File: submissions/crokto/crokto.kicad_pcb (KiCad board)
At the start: 2 copper layers, 88.9 x 50 mm, 27 parts, among them J1 USB_C_Receptacle, K1 UP, K3 LEFT, K4 RIGHT, K6 A, K7 DOWN, K8 B, SW1 SW_PUSH, SW2 SELECT, SW3 START, U1 ATmega32U2-AU, Y1 Resonator

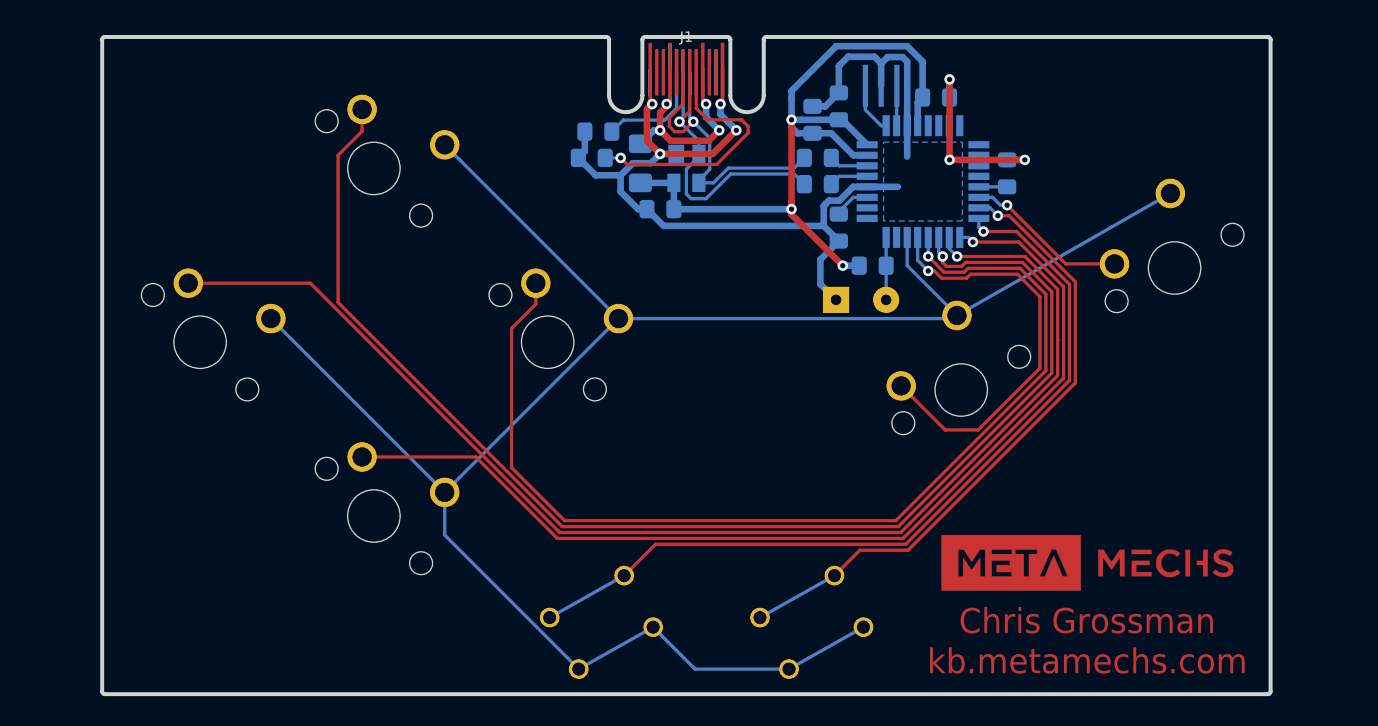
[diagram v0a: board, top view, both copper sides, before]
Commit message: switched design entirely lol
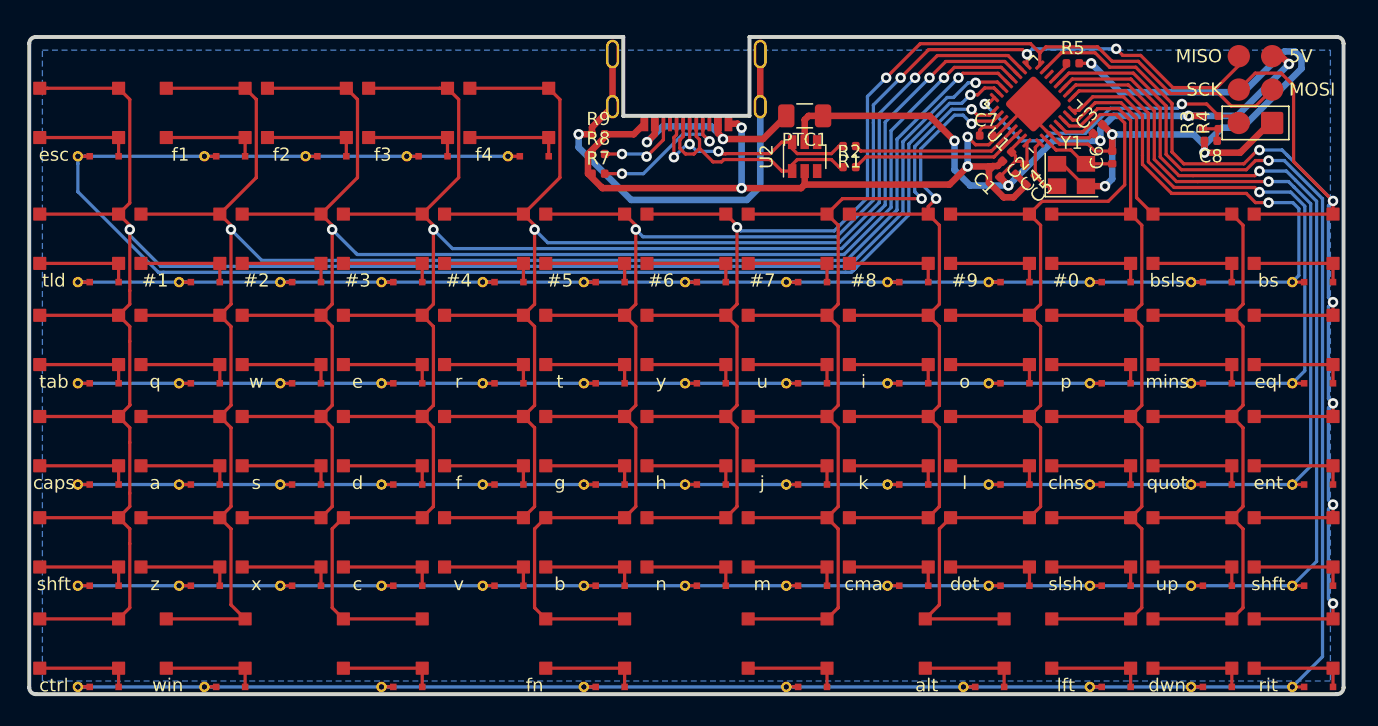
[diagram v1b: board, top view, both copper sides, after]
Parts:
- removed G***: LOGO, logo:qr
- removed L1: MountingHole, logo:new logo
- removed R6: 5.1k, Resistor_SMD:R_0805_2012Metric_Pad1.15x1.40mm_HandSolder
- removed SW1: SW_PUSH, Connector_Wire:SolderWirePad_1x02_P3.81mm_Drill0.8mm
- removed SW2: SELECT, crokto:FSMJ_2-1825910-7
- removed SW3: START, crokto:FSMJ_2-1825910-7
- added C6: 10pf, Capacitor_SMD:C_0402_1005Metric, F.Cu at (82.4, 9.16)
- added C7: 1u, Capacitor_SMD:C_0402_1005Metric, F.Cu at (72.8, 7.50)
- added C8: 100n, Capacitor_SMD:C_0402_1005Metric, F.Cu at (89.9, 7.90)
- added D10: D, crokto:D_SOD-323F-VIA, F.Cu at (36.5, 18.6)
- added D11: D, crokto:D_SOD-323F-VIA, F.Cu at (44.2, 18.6)
- added D12: D, crokto:D_SOD-323F-VIA, F.Cu at (51.9, 18.6)
- added D13: D, crokto:D_SOD-323F-VIA, F.Cu at (59.6, 18.6)
- added D14: D, crokto:D_SOD-323F-VIA, F.Cu at (67.3, 18.6)
- added D15: D, crokto:D_SOD-323F-VIA, F.Cu at (75.0, 18.6)
- added D16: D, crokto:D_SOD-323F-VIA, F.Cu at (82.7, 18.6)
- added D17: D, crokto:D_SOD-323F-VIA, F.Cu at (90.4, 18.6)
- added D18: D, crokto:D_SOD-323F-VIA, F.Cu at (98.1, 18.6)
- added D19: D, crokto:D_SOD-323F-VIA, F.Cu at (5.70, 26.4)
- added D2: D, crokto:D_SOD-323F-VIA, F.Cu at (15.3, 9.07)
- added D20: D, crokto:D_SOD-323F-VIA, F.Cu at (13.4, 26.4)
- added D21: D, crokto:D_SOD-323F-VIA, F.Cu at (21.1, 26.4)
- added D22: D, crokto:D_SOD-323F-VIA, F.Cu at (28.8, 26.4)
- added D23: D, crokto:D_SOD-323F-VIA, F.Cu at (36.5, 26.4)
- added D24: D, crokto:D_SOD-323F-VIA, F.Cu at (44.2, 26.4)
- added D25: D, crokto:D_SOD-323F-VIA, F.Cu at (51.9, 26.4)
- added D26: D, crokto:D_SOD-323F-VIA, F.Cu at (59.6, 26.4)
- added D27: D, crokto:D_SOD-323F-VIA, F.Cu at (67.3, 26.4)
- added D28: D, crokto:D_SOD-323F-VIA, F.Cu at (75.0, 26.4)
- added D29: D, crokto:D_SOD-323F-VIA, F.Cu at (82.7, 26.4)
- added D3: D, crokto:D_SOD-323F-VIA, F.Cu at (23.0, 9.07)
- added D30: D, crokto:D_SOD-323F-VIA, F.Cu at (90.4, 26.4)
- added D31: D, crokto:D_SOD-323F-VIA, F.Cu at (98.1, 26.4)
- added D32: D, crokto:D_SOD-323F-VIA, F.Cu at (5.70, 34.0)
- added D33: D, crokto:D_SOD-323F-VIA, F.Cu at (13.4, 34.0)
- added D34: D, crokto:D_SOD-323F-VIA, F.Cu at (21.1, 34.0)
- added D35: D, crokto:D_SOD-323F-VIA, F.Cu at (28.8, 34.0)
- added D36: D, crokto:D_SOD-323F-VIA, F.Cu at (36.5, 34.0)
- added D37: D, crokto:D_SOD-323F-VIA, F.Cu at (44.2, 34.0)
- added D38: D, crokto:D_SOD-323F-VIA, F.Cu at (51.9, 34.0)
- added D39: D, crokto:D_SOD-323F-VIA, F.Cu at (59.6, 34.0)
- added D4: D, crokto:D_SOD-323F-VIA, F.Cu at (30.7, 9.07)
- added D40: D, crokto:D_SOD-323F-VIA, F.Cu at (67.3, 34.0)
- added D41: D, crokto:D_SOD-323F-VIA, F.Cu at (75.0, 34.0)
- added D42: D, crokto:D_SOD-323F-VIA, F.Cu at (82.7, 34.0)
- added D43: D, crokto:D_SOD-323F-VIA, F.Cu at (90.4, 34.0)
- added D44: D, crokto:D_SOD-323F-VIA, F.Cu at (98.1, 34.0)
- added D45: D, crokto:D_SOD-323F-VIA, F.Cu at (5.70, 41.8)
- added D46: D, crokto:D_SOD-323F-VIA, F.Cu at (13.4, 41.8)
- added D47: D, crokto:D_SOD-323F-VIA, F.Cu at (21.1, 41.8)
- added D48: D, crokto:D_SOD-323F-VIA, F.Cu at (28.8, 41.8)
- added D49: D, crokto:D_SOD-323F-VIA, F.Cu at (36.5, 41.8)
- added D5: D, crokto:D_SOD-323F-VIA, F.Cu at (38.4, 9.07)
- added D50: D, crokto:D_SOD-323F-VIA, F.Cu at (44.2, 41.8)
- added D51: D, crokto:D_SOD-323F-VIA, F.Cu at (51.9, 41.8)
- added D52: D, crokto:D_SOD-323F-VIA, F.Cu at (59.6, 41.8)
- added D53: D, crokto:D_SOD-323F-VIA, F.Cu at (67.3, 41.8)
- added D54: D, crokto:D_SOD-323F-VIA, F.Cu at (75.0, 41.8)
- added D55: D, crokto:D_SOD-323F-VIA, F.Cu at (82.7, 41.8)
- added D56: D, crokto:D_SOD-323F-VIA, F.Cu at (90.4, 41.8)
- added D57: D, crokto:D_SOD-323F-VIA, F.Cu at (98.1, 41.8)
- added D58: D, crokto:D_SOD-323F-VIA, F.Cu at (5.70, 49.5)
- added D59: D, crokto:D_SOD-323F-VIA, F.Cu at (15.3, 49.5)
- added D6: D, crokto:D_SOD-323F-VIA, F.Cu at (5.70, 18.6)
- added D60: D, crokto:D_SOD-323F-VIA, F.Cu at (28.8, 49.5)
- added D61: D, crokto:D_SOD-323F-VIA, F.Cu at (44.2, 49.5)
- added D62: D, crokto:D_SOD-323F-VIA, F.Cu at (59.6, 49.5)
- added D63: D, crokto:D_SOD-323F-VIA, F.Cu at (73.1, 49.5)
- added D64: D, crokto:D_SOD-323F-VIA, F.Cu at (82.7, 49.5)
- added D65: D, crokto:D_SOD-323F-VIA, F.Cu at (90.4, 49.5)
- added D66: D, crokto:D_SOD-323F-VIA, F.Cu at (98.1, 49.5)
- added D7: D, crokto:D_SOD-323F-VIA, F.Cu at (13.4, 18.6)
- added D8: D, crokto:D_SOD-323F-VIA, F.Cu at (21.1, 18.6)
- added D9: D, crokto:D_SOD-323F-VIA, F.Cu at (28.8, 18.6)
- added H1: logo, logo:100mm wide logo, B.Cu at (51.8, 40.8)
- added H2: logo, logo:qr, B.Cu at (7.00, 7.00)
- added K10: #4, smd-keys:100, F.Cu at (34.6, 15.3)
- added K11: #5, smd-keys:100, F.Cu at (42.3, 15.3)
- added K12: #6, smd-keys:100, F.Cu at (50.0, 15.3)
- added K13: #7, smd-keys:100, F.Cu at (57.7, 15.3)
- added K14: #8, smd-keys:100, F.Cu at (65.4, 15.3)
- added K15: #9, smd-keys:100, F.Cu at (73.1, 15.3)
- added K16: #0, smd-keys:100, F.Cu at (80.8, 15.3)
- added K17: bsls, smd-keys:100, F.Cu at (88.5, 15.3)
- added K18: bs, smd-keys:100, F.Cu at (96.2, 15.3)
- added K19: tab, smd-keys:100, F.Cu at (3.80, 23.1)
- added K2: f1, smd-keys:100, F.Cu at (13.4, 5.78)
- added K20: q, smd-keys:100, F.Cu at (11.5, 23.1)
- added K21: w, smd-keys:100, F.Cu at (19.2, 23.1)
- added K22: e, smd-keys:100, F.Cu at (26.9, 23.1)
- added K23: r, smd-keys:100, F.Cu at (34.6, 23.1)
- added K24: t, smd-keys:100, F.Cu at (42.3, 23.1)
- added K25: y, smd-keys:100, F.Cu at (50.0, 23.1)
- added K26: u, smd-keys:100, F.Cu at (57.7, 23.1)
- added K27: i, smd-keys:100, F.Cu at (65.4, 23.1)
- added K28: o, smd-keys:100, F.Cu at (73.1, 23.1)
- added K29: p, smd-keys:100, F.Cu at (80.8, 23.1)
- added K30: mins, smd-keys:100, F.Cu at (88.5, 23.1)
- added K31: eql, smd-keys:100, F.Cu at (96.2, 23.1)
- added K32: caps, smd-keys:100, F.Cu at (3.80, 30.8)
- added K33: a, smd-keys:100, F.Cu at (11.5, 30.8)
- added K34: s, smd-keys:100, F.Cu at (19.2, 30.8)
- added K35: d, smd-keys:100, F.Cu at (26.9, 30.8)
- added K36: f, smd-keys:100, F.Cu at (34.6, 30.8)
- added K37: g, smd-keys:100, F.Cu at (42.3, 30.8)
- added K38: h, smd-keys:100, F.Cu at (50.0, 30.8)
- added K39: j, smd-keys:100, F.Cu at (57.7, 30.8)
- added K40: k, smd-keys:100, F.Cu at (65.4, 30.8)
- added K41: l, smd-keys:100, F.Cu at (73.1, 30.8)
- added K42: clns, smd-keys:100, F.Cu at (80.8, 30.8)
- added K43: quot, smd-keys:100, F.Cu at (88.5, 30.8)
- added K44: ent, smd-keys:100, F.Cu at (96.2, 30.8)
- added K45: shft, smd-keys:100, F.Cu at (3.80, 38.5)
- added K46: z, smd-keys:100, F.Cu at (11.5, 38.5)
- added K47: x, smd-keys:100, F.Cu at (19.2, 38.5)
- added K48: c, smd-keys:100, F.Cu at (26.9, 38.5)
- added K49: v, smd-keys:100, F.Cu at (34.6, 38.5)
- added K5: f4, smd-keys:100, F.Cu at (36.5, 5.78)
- added K50: b, smd-keys:100, F.Cu at (42.3, 38.5)
- added K51: n, smd-keys:100, F.Cu at (50.0, 38.5)
- added K52: m, smd-keys:100, F.Cu at (57.7, 38.5)
- added K53: cma, smd-keys:100, F.Cu at (65.4, 38.5)
- added K54: dot, smd-keys:100, F.Cu at (73.1, 38.5)
- added K55: slsh, smd-keys:100, F.Cu at (80.8, 38.5)
- added K56: up, smd-keys:100, F.Cu at (88.5, 38.5)
- added K57: shft, smd-keys:100, F.Cu at (96.2, 38.5)
- added K58: ctrl, smd-keys:100, F.Cu at (3.80, 46.1)
- added K59: win, smd-keys:150, F.Cu at (13.4, 46.1)
- added K60: , smd-keys:200, F.Cu at (26.9, 46.1)
- added K61: fn, smd-keys:200, F.Cu at (42.3, 46.1)
- added K62: , smd-keys:200, F.Cu at (57.7, 46.1)
- added K63: alt, smd-keys:150, F.Cu at (71.2, 46.1)
- added K64: lft, smd-keys:100, F.Cu at (80.8, 46.1)
- added K65: dwn, smd-keys:100, F.Cu at (88.5, 46.1)
- added K66: rit, smd-keys:100, F.Cu at (96.2, 46.1)
- added K9: #3, smd-keys:100, F.Cu at (26.9, 15.3)
- added R7: 5.1k, Resistor_SMD:R_0402_1005Metric, F.Cu at (43.3, 10.4)
- added R8: 5.1k, Resistor_SMD:R_0402_1005Metric, F.Cu at (43.3, 8.90)
- added R9: 0, Resistor_SMD:R_0402_1005Metric, F.Cu at (43.3, 7.40)
- added U2: SRV05-4, Package_TO_SOT_SMD:SOT-23-6, F.Cu at (59.0, 9.10)
- added USB1: HRO-TYPE-C-31-M-12, Type-C:HRO-TYPE-C-31-M-13, F.Cu at (50.0, -0.80)
- C1, C2, C3, C4: footprint Capacitor_SMD:C_0805_2012Metric_Pad1.15x1.40mm_HandSolder -> Capacitor_SMD:C_0402_1005Metric; moved to F.Cu
- C5: value 1u -> 10pf; footprint Capacitor_SMD:C_0805_2012Metric_Pad1.15x1.40mm_HandSolder -> Capacitor_SMD:C_0402_1005Metric; moved to F.Cu
- D1: value PRTR5V0U2X -> D; footprint Package_TO_SOT_SMD:SOT-143 -> crokto:D_SOD-323F-VIA; moved to F.Cu
- J1: value USB_C_Receptacle -> AVR-ISP-6; footprint pcb-usb:USB_TYPE_C_DS_5 -> crokto:2x3-jumper
- K1: value UP -> esc; footprint switches-nocopper:MX-100 -> smd-keys:100
- K3: value LEFT -> f2; footprint switches-nocopper:MX-100 -> smd-keys:100
- K4: value RIGHT -> f3; footprint switches-nocopper:MX-100 -> smd-keys:100
- K6: value A -> tld; footprint switches-nocopper:MX-100 -> smd-keys:100
- K7: value DOWN -> #1; footprint switches-nocopper:MX-100 -> smd-keys:100
- K8: value B -> #2; footprint switches-nocopper:MX-100 -> smd-keys:100
- PTC1: footprint Fuse:Fuse_1206_3216Metric_Pad1.42x1.75mm_HandSolder -> Fuse:Fuse_1206_3216Metric; moved to F.Cu
- R1: value 10k -> 22; footprint Resistor_SMD:R_0805_2012Metric_Pad1.15x1.40mm_HandSolder -> Resistor_SMD:R_0402_1005Metric; moved to F.Cu
- R2: footprint Resistor_SMD:R_0805_2012Metric_Pad1.15x1.40mm_HandSolder -> Resistor_SMD:R_0402_1005Metric; moved to F.Cu
- R3: value 22 -> 4.7K; footprint Resistor_SMD:R_0805_2012Metric_Pad1.15x1.40mm_HandSolder -> Resistor_SMD:R_0402_1005Metric; moved to F.Cu
- R4: value 10k -> 330; footprint Resistor_SMD:R_0805_2012Metric_Pad1.15x1.40mm_HandSolder -> Resistor_SMD:R_0402_1005Metric; moved to F.Cu
- R5: value 5.1k -> 10k; footprint Resistor_SMD:R_0805_2012Metric_Pad1.15x1.40mm_HandSolder -> Resistor_SMD:R_0402_1005Metric; moved to F.Cu
- U1: value ATmega32U2-AU -> ATmega16U2-MU; footprint Package_QFP:TQFP-32_7x7mm_P0.8mm -> Package_DFN_QFN:QFN-32-1EP_5x5mm_P0.5mm_EP3.1x3.1mm; moved to F.Cu
- Y1: value Resonator -> Crystal_GND24; footprint Crystal:Resonator_SMD_muRata_CSTxExxV-3Pin_3.0x1.1mm_HandSoldering -> Crystal:Crystal_SMD_3225-4Pin_3.2x2.5mm; moved to F.Cu
- moved K6 83.4 mm to (3.80, 15.3), turned to 180 degrees
- moved K8 53.0 mm to (19.2, 15.3), turned to 180 degrees
- moved D1 44.3 mm to (5.70, 9.07), turned to 0 degrees
- moved J1 43.5 mm to (93.3, 4.00)
- moved R5 37.3 mm to (79.4, 2.00)
- moved R3 29.4 mm to (89.3, 6.50), turned to 90 degrees
- moved K7 25.7 mm to (11.5, 15.3), turned to 180 degrees
- moved C1 25.6 mm to (73.5, 10.3), turned to 135 degrees
- moved K1 22.8 mm to (3.80, 5.78), turned to 180 degrees
- moved K4 20.4 mm to (28.8, 5.78), turned to 180 degrees
- moved C3 19.8 mm to (81.3, 7.00), turned to 45 degrees
- moved K3 19.2 mm to (21.1, 5.78), turned to 180 degrees
- moved R4 16.6 mm to (90.5, 6.50), turned to 90 degrees
- moved Y1 16.0 mm to (79.3, 10.5)
- moved C2 15.1 mm to (74.4, 9.10), turned to 225 degrees
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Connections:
- C1 pad 1: VCC -> +5V
- C2 pad 1: VCC -> +5V
- C3 pad 1: VCC -> +5V
- C4 pad 1: VCC -> +5V
- C5 pad 1: GND -> Net-(C5-Pad1)
- C5 pad 2: Net-(C5-Pad2) -> GND
- D1 pad 1: GND -> /16u2/C6
- D1 pad 2: /DB+ -> Net-(D1-Pad2)
- K1 pad 1: /c -> Net-(D1-Pad2)
- K1 pad 2: /up -> /16u2/C7
- K3 pad 1: /c -> Net-(D3-Pad2)
- K3 pad 2: /left -> /16u2/B6
- K4 pad 1: /c -> Net-(D4-Pad2)
- K4 pad 2: /right -> /16u2/B5
- K6 pad 1: /c -> Net-(D6-Pad2)
- K6 pad 2: /a -> /16u2/C7
- K7 pad 1: /c -> Net-(D7-Pad2)
- K7 pad 2: /down -> /16u2/B7
- K8 pad 1: /c -> Net-(D8-Pad2)
- K8 pad 2: /b -> /16u2/B6
- PTC1 pad 1: VCC -> +5V
- R1 pad 1: Net-(R1-Pad1) -> /16u2/D+
- R1 pad 2: VCC -> /16u2/DB+
- R2 pad 1: /D+ -> /16u2/DB-
- R2 pad 2: /DB+ -> /16u2/D-
- R3 pad 1: /DB- -> Net-(C8-Pad1)
- R3 pad 2: /D- -> +5V
- R4 pad 1: GND -> Net-(C8-Pad1)
- R4 pad 2: Net-(R4-Pad2) -> /16u2/RST
- R5 pad 1: GND -> Net-(R5-Pad1)
- R5 pad 2: Net-(J1-PadA5) -> GND
- U1 pad 1: Net-(U1-Pad1) -> Net-(C5-Pad1)
- U1 pad 10: (no net) -> /16u2/D4
- U1 pad 11: (no net) -> /16u2/D5
- U1 pad 12: (no net) -> /16u2/D6
- U1 pad 13: Net-(R4-Pad2) -> Net-(R5-Pad1)
- U1 pad 14: /a -> (no net)
- U1 pad 15: /start -> /16u2/B1
- U1 pad 16: /select -> /16u2/B2
- U1 pad 17: /down -> /16u2/B3
- U1 pad 18: /left -> /16u2/B4
- U1 pad 19: /up -> /16u2/B5
- U1 pad 20: /right -> /16u2/B6
- U1 pad 21: /b -> /16u2/B7
- U1 pad 22: /c -> /16u2/C7
- U1 pad 23: (no net) -> /16u2/C6
- U1 pad 24: Net-(R1-Pad1) -> /16u2/RST
- U1 pad 25: (no net) -> /16u2/C5
- U1 pad 26: (no net) -> /16u2/C4
- U1 pad 27: Net-(C5-Pad2) -> Net-(C7-Pad1)
- U1 pad 29: /D+ -> /16u2/D+
- U1 pad 30: /D- -> /16u2/D-
- U1 pad 31: VCC -> +5V
- U1 pad 32: VCC -> +5V
- U1 pad 4: VCC -> +5V
- U1 pad 5: (no net) -> /16u2/C2
- U1 pad 6: (no net) -> /16u2/D0
- U1 pad 7: (no net) -> /16u2/D1
- U1 pad 8: (no net) -> /16u2/D2
- U1 pad 9: (no net) -> /16u2/D3
- Y1 pad 1: Net-(U1-Pad1) -> Net-(C5-Pad1)
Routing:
- net /16u2/D6: track 0.00 -> 165.7 mm, vias 0 -> 1
- net /16u2/D5: track 0.00 -> 160.0 mm, vias 0 -> 1
- net /16u2/C7: track 0.00 -> 157.0 mm, vias 0 -> 2
- net /16u2/D4: track 0.00 -> 150.7 mm, vias 0 -> 1
- net /c: track 150.5 -> 0.00 mm
- net /16u2/B7: track 0.00 -> 150.3 mm, vias 0 -> 2
- net /16u2/D3: track 0.00 -> 141.7 mm, vias 0 -> 1
- net /16u2/B5: track 0.00 -> 135.8 mm, vias 0 -> 2
- net /16u2/D2: track 0.00 -> 133.3 mm, vias 0 -> 1
- net /16u2/B6: track 0.00 -> 128.6 mm, vias 0 -> 2
- net /16u2/B3: track 0.00 -> 123.7 mm, vias 0 -> 4
- net /16u2/C6: track 0.00 -> 122.0 mm, vias 0 -> 1
- net /16u2/B4: track 0.00 -> 114.1 mm, vias 0 -> 2
- net /16u2/B1: track 0.00 -> 112.5 mm, vias 0 -> 6
- net /16u2/B2: track 0.00 -> 104.4 mm, vias 0 -> 2
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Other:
- board size 88.9 x 50 mm -> 100 x 50 mm
- board text added: "Chris Grossman Keyboard Designer crokto@metamechs.com kb.metamechs.com"
- board text removed: "Chris Grossman kb.metamechs.com"
- board text removed: "JLCJLCJLCJLC"
